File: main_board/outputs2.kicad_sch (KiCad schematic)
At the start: 25 parts, among them U15 CJ431, U5 TL072CDR, U7 TL072CDR

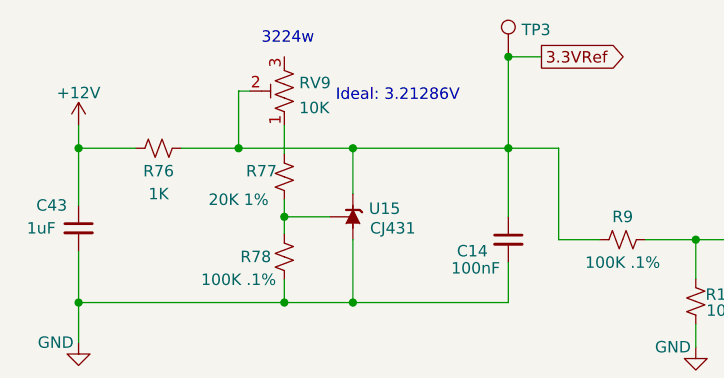
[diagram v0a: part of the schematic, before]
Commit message: After project cleanup
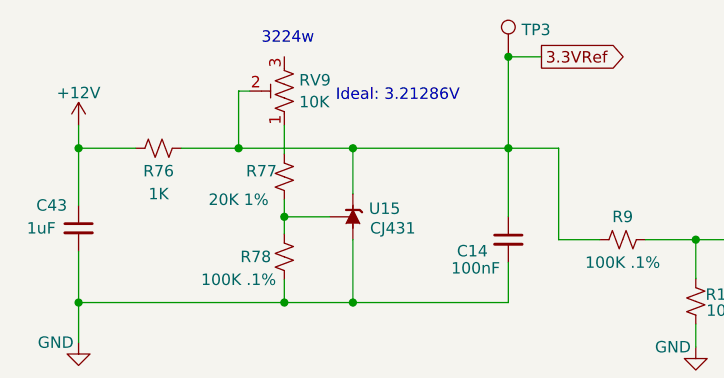
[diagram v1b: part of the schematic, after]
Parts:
- RV9: footprint Potentiometer_SMD:Potentiometer_Bourns_3224W_Vertical -> greenface:Potentiometer_Bourns_3224W_Vertical
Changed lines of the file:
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@@
 		(fields_autoplaced yes)
 		(property "Reference" "RV9"
-			(at 54.991 26.5235 0)
+			(at 54.991 26.2198 0)
 			(effects
 				(font
@@
 		)
 		(property "Value" "10K"
-			(at 54.991 29.2986 0)
+			(at 54.991 28.6441 0)
 			(effects
 				(font
@@
 			)
 		)
-		(property "Footprint" "Potentiometer_SMD:Potentiometer_Bourns_3224W_Vertical"
+		(property "Footprint" "greenface:Potentiometer_Bourns_3224W_Vertical"
 			(at 53.34 27.432 0)
 			(effects
